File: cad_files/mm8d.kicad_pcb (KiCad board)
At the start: 2 copper layers, 81 parts, among them J1 Screw_Terminal_1x05, J10 Screw_Terminal_1x05, J2 Screw_Terminal_1x04, J3 Screw_Terminal_1x04, J4 Screw_Terminal_1x04, J5 Screw_Terminal_1x04, J6 Screw_Terminal_1x03, J7 Screw_Terminal_1x03, J8 Screw_Terminal_1x03, J9 Screw_Terminal_1x03, K1 LEG-5, K2 LEG-5, K3 LEG-5, K4 LEG-5, Q1 BC548C, Q2 BC548C, Q3 BC548C, Q4 BC548C, Q5 BC548C, Q6 BC548C, Q7 BC548C, Q8 BC548C, U1 4N25, U2 4N25, U3 4N25, U4 4N25, U5 74LS14, U6 74LS05

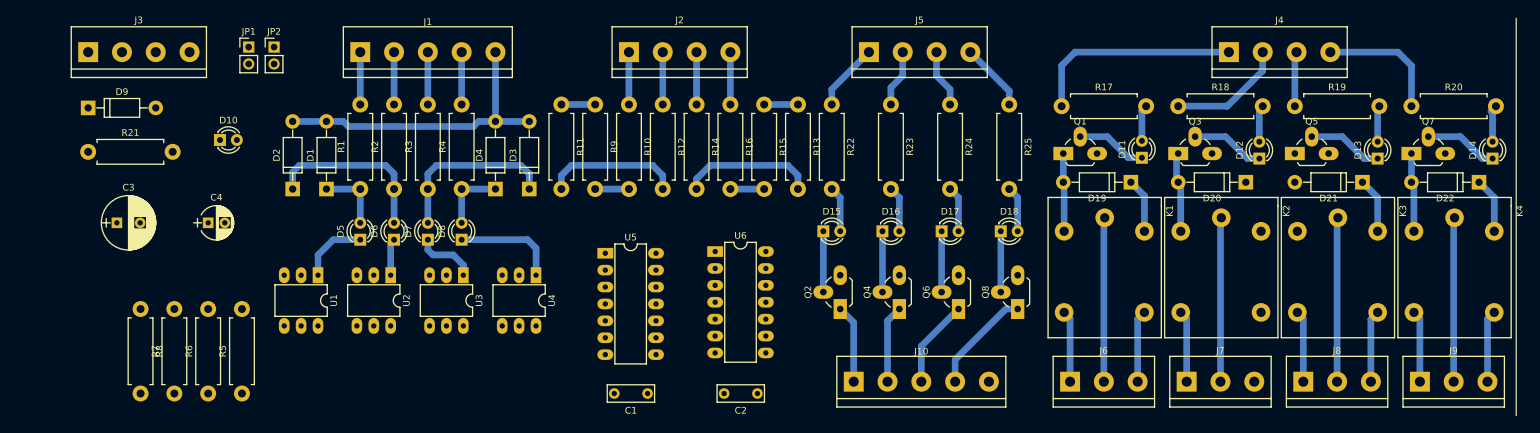
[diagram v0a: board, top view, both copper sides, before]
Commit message: 210305
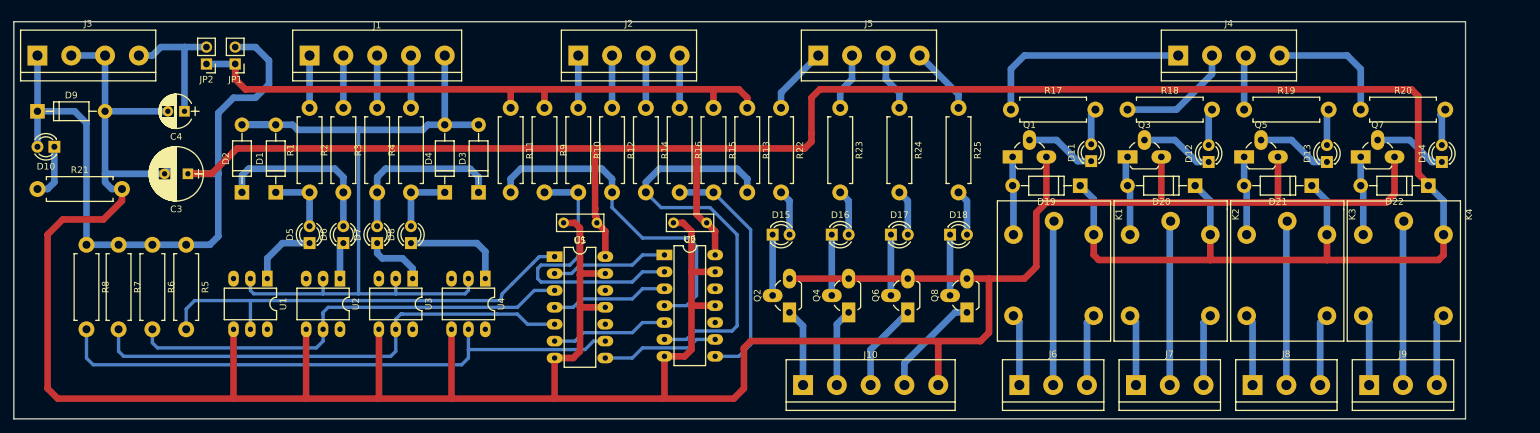
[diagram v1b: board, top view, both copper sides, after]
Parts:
- moved C1 26.8 mm to (127.8, 98.6)
- moved C2 26.8 mm to (144.3, 98.6)
- moved D10 24.9 mm to (46.2, 87.1), turned to 180 degrees
- moved R5 23.9 mm to (66.0, 101.9), turned to 270 degrees
- moved R6 23.9 mm to (61.0, 101.9), turned to 270 degrees
- moved R7 23.9 mm to (55.9, 101.9), turned to 270 degrees
- moved C4 17.1 mm to (65.8, 81.8), turned to 180 degrees
- moved C3 13.0 mm to (66.3, 91.2), turned to 180 degrees
- moved R8 12.6 mm to (51.1, 101.9)
- moved JP2 10.5 mm to (69.1, 74.7), turned to 180 degrees
- moved R21 9.45 mm to (43.7, 93.5)
- moved D22 7.64 mm to (252.7, 93.0)
- moved K4 7.64 mm to (248.9, 106.4)
- moved D1 7.64 mm to (79.5, 94.0)
- moved D11 7.64 mm to (202.1, 89.3)
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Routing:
- net GND: track 0.00 -> 496.1 mm
- net VCC: track 24.8 -> 444.5 mm
- net Net-(R8-Pad2): track 0.00 -> 88.0 mm
- net Net-(JP1-Pad1): track 10.2 -> 94.6 mm
- net Net-(R7-Pad2): track 0.00 -> 75.5 mm
- net Net-(D1-Pad2): track 46.6 -> 117.6 mm
- net Net-(R6-Pad2): track 0.00 -> 68.9 mm
- net Net-(R5-Pad2): track 0.00 -> 66.4 mm
- net Net-(R13-Pad2): track 20.3 -> 62.1 mm
- net Net-(R10-Pad2): track 5.08 -> 43.0 mm
- net Net-(R15-Pad2): track 5.08 -> 36.3 mm
- net Net-(R11-Pad2): track 20.6 -> 50.8 mm
- net Net-(C4-Pad1): track 0.00 -> 20.6 mm
- net Net-(U5-Pad8): track 0.00 -> 17.7 mm
- net Net-(U5-Pad4): track 0.00 -> 17.7 mm
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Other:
- board outline added: 218.2 x 59.7 mm
